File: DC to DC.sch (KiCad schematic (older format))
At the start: 27 parts, among them J10 Screw_Terminal_01x02, U16 L4971, U17 LM1117-5.0, U18 LM1117-3.3

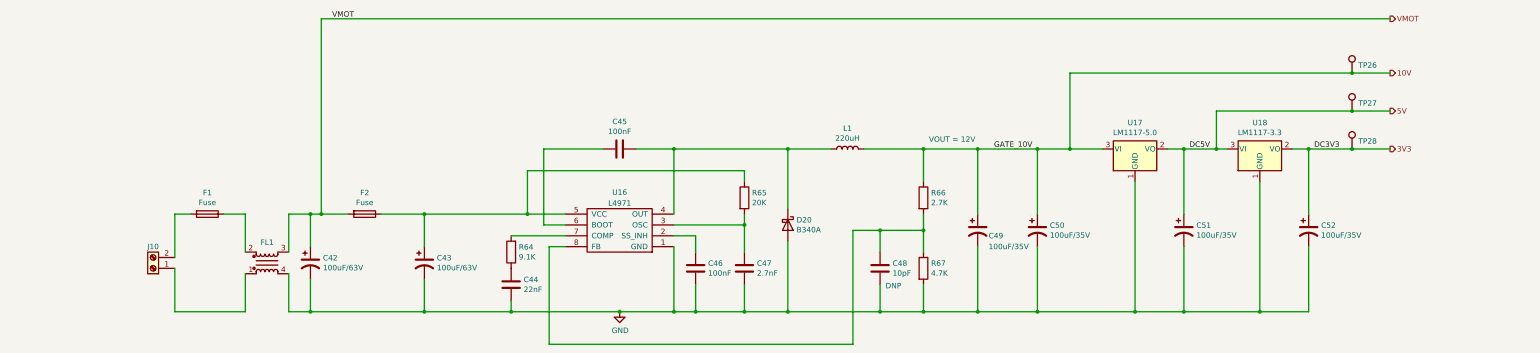
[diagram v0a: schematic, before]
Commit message: 0503_2021_Update
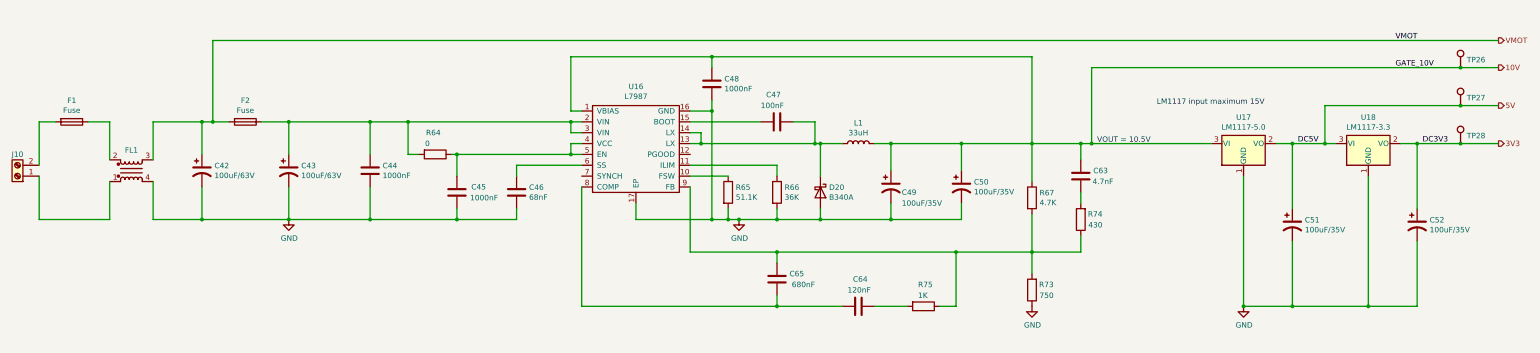
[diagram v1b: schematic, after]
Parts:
- removed U16: L4971, Package_DIP:DIP-8_W7.62mm_LongPads, symbol dc_to_dc:L4971
- added C63: 4.7nF, Capacitor_SMD:C_0603_1608Metric_Pad1.08x0.95mm_HandSolder, symbol Device:C
- added C64: 120nF, Capacitor_SMD:C_0603_1608Metric_Pad1.08x0.95mm_HandSolder, symbol Device:C
- added C65: 680nF, Capacitor_SMD:C_0603_1608Metric_Pad1.08x0.95mm_HandSolder, symbol Device:C
- added R73: 750, Resistor_SMD:R_0603_1608Metric_Pad0.98x0.95mm_HandSolder, symbol Device:R
- added R74: 430, Resistor_SMD:R_0603_1608Metric_Pad0.98x0.95mm_HandSolder, symbol Device:R
- added R75: 1K, Resistor_SMD:R_0603_1608Metric_Pad0.98x0.95mm_HandSolder, symbol Device:R
- added U16: L7987, Package_SO:HTSSOP-16-1EP_4.4x5mm_P0.65mm_EP3x3mm, symbol dc_to_dc:L7987
- C44: value 22nF -> 1000nF
- C45: value 100nF -> 1000nF
- C46: value 100nF -> 68nF
- C47: value 2.7nF -> 100nF
- C48: value 10pF -> 1000nF
- L1: value 220uH -> 33uH
- R64: value 9.1K -> 0
- R65: value 20K -> 51.1K
- R66: value 2.7K -> 36K; footprint Resistor_SMD:R_1206_3216Metric_Pad1.30x1.75mm_HandSolder -> Resistor_SMD:R_0603_1608Metric_Pad0.98x0.95mm_HandSolder
- R67: footprint Resistor_SMD:R_1206_3216Metric_Pad1.30x1.75mm_HandSolder -> Resistor_SMD:R_0603_1608Metric_Pad0.98x0.95mm_HandSolder
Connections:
- net 10V: now also C48.1, R67.1, C63.2, U16.1 (VBIAS); no longer R66.1
- net GND: now also C45.1, R65.2, R66.2, R73.1, U16.16 (GND), U16.17 (EP); no longer C47.2, R67.2
- net at C46.1: now also U16.6 (SS)
- net at C47.1: now also D20.1 (K), L1.1, U16.13 (LX), U16.14 (LX); no longer R65.2
- net at C43.1, F2.1: now also C44.1, R64.2, U16.2 (VIN), U16.3 (VIN); no longer R65.1
- net at C45.2: now also R64.1, U16.4 (VCC), U16.5 (EN)
- new net: R65.1, U16.10 (FSW)
- new net: C47.2, U16.15 (BOOT)
- new net: R66.1, U16.11 (ILIM)
- new net: C65.2, R67.2, R73.2, R74.1, R75.1, U16.9 (FB)
- new net: C64.2, C65.1, U16.8 (COMP)
- new net: C63.1, R74.2
- new net: C64.1, R75.2
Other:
- note added: "LM1117 input maximum 15V"
- note added: "VOUT = 10.5V"
- note removed: "DNP"
- note removed: "VOUT = 12V"
- moved on the sheet: C42, C43, C44, C45, C46, C47, C48, C49, C50, C51, C52, D20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
